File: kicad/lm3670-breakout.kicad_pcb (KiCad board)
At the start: 2 copper layers, 17 x 10.5 mm, 7 parts

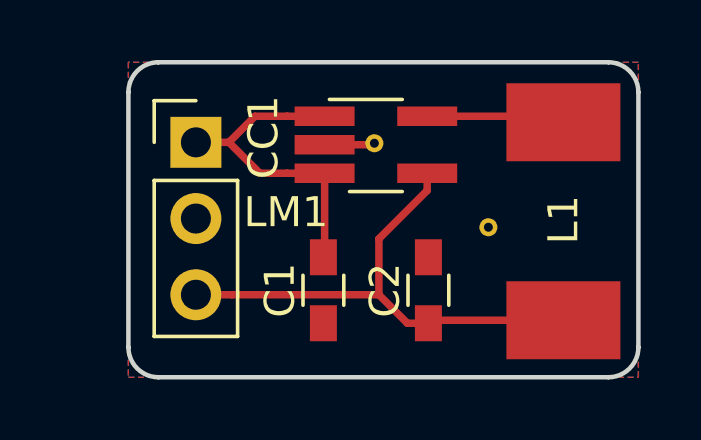
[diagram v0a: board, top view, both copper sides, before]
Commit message: updated pcb
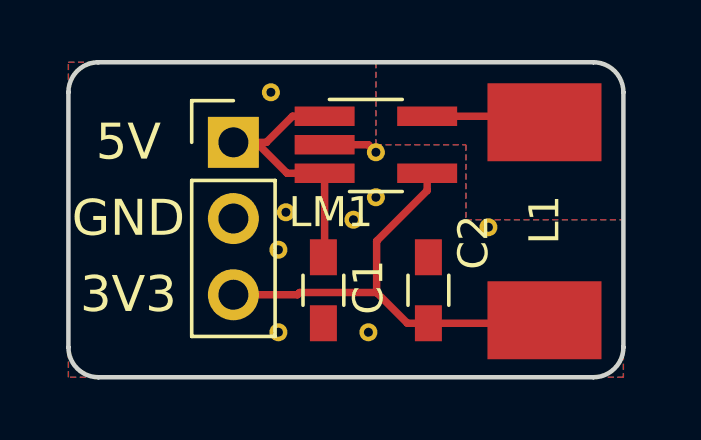
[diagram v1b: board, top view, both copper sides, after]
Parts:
- added REF**: STITCHING_VIA, utils:STITCHING_VIA, F.Cu at (144.5, 111.5)
- added REF**: STITCHING_VIA, utils:STITCHING_VIA, F.Cu at (141.5, 111.5)
- added REF**: STITCHING_VIA, utils:STITCHING_VIA, F.Cu at (144.0, 107.8)
- added REF**: STITCHING_VIA, utils:STITCHING_VIA, F.Cu at (141.2, 103.5)
- added REF**: STITCHING_VIA, utils:STITCHING_VIA, F.Cu at (141.5, 108.8)
- added REF**: STITCHING_VIA, utils:STITCHING_VIA, F.Cu at (141.8, 107.5)
- added REF**: STITCHING_VIA, utils:STITCHING_VIA, F.Cu at (144.8, 107.0)
- moved CC1 1.25 mm to (140.0, 105.2)
- moved L1 0.63 mm to (150.4, 107.8)
- moved REF** 0.30 mm to (144.8, 105.5)
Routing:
- net /3V3: track 17.4 -> 15.5 mm
- net /5V: track 11.1 -> 9.68 mm
- net Net-(L1-Pad2): track 4.62 -> 3.99 mm
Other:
- board size 17 x 10.5 mm -> 18.5 x 10.5 mm
- net class Default: clearance 0.2 -> 0.3; via_dia 0.6 -> 0.45; via_drill 0.4 -> 0.2
- rule trace_clearance: 0.2 -> 0.3
- rule via_min_drill: 0.3 -> 0.2
- rule via_min_size: 0.4 -> 0.45
- board text added: "3V3"
- board text added: "5V"
- board text added: "GND"
- board text added: "hochreiner.net lm3670-breakout V1.0.1"
- board text added: "max 350 mA"
